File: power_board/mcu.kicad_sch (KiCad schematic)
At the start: 23 parts, among them J1 Conn_ARM_SWD_TagConnect_TC203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, U15 SM05B-GHS-TB(LF)(SN), U2 LM66100DCKR, U3 STM32L431KCUx

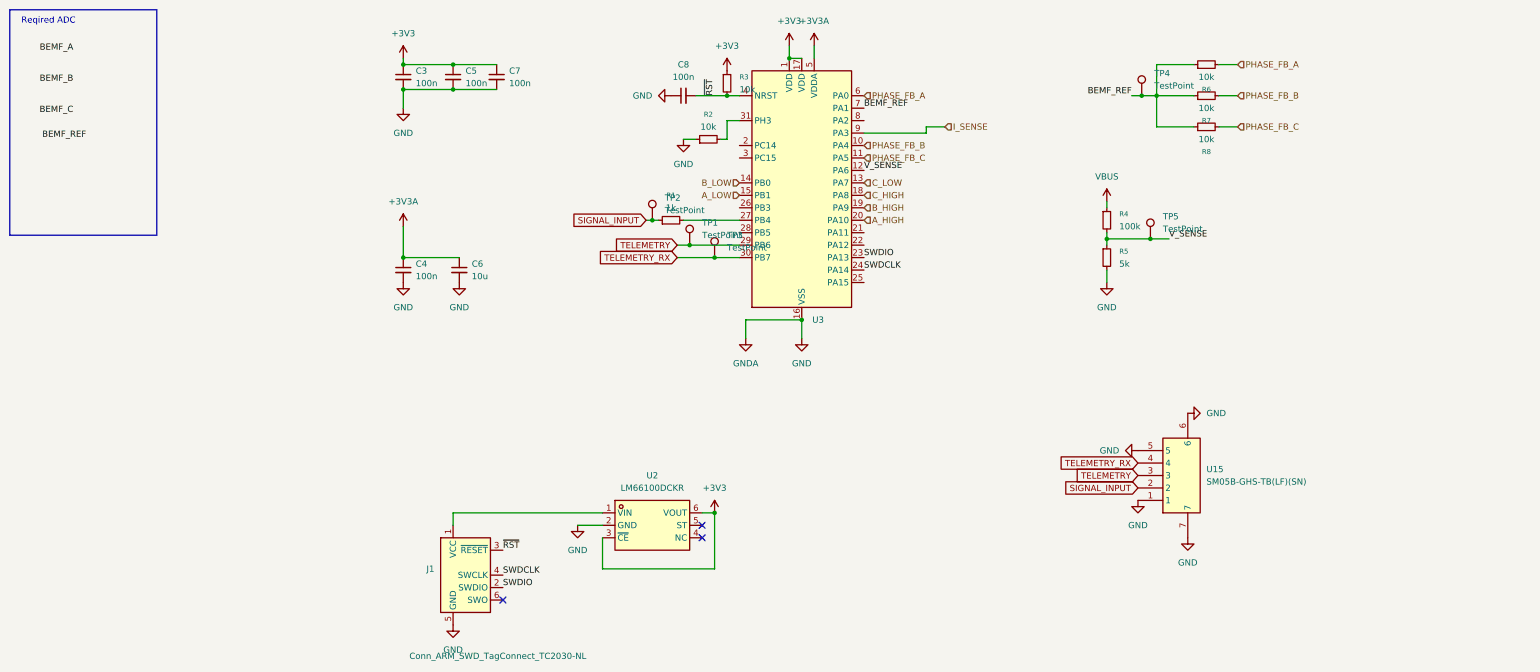
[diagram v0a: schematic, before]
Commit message: Complete all design, pass DRC
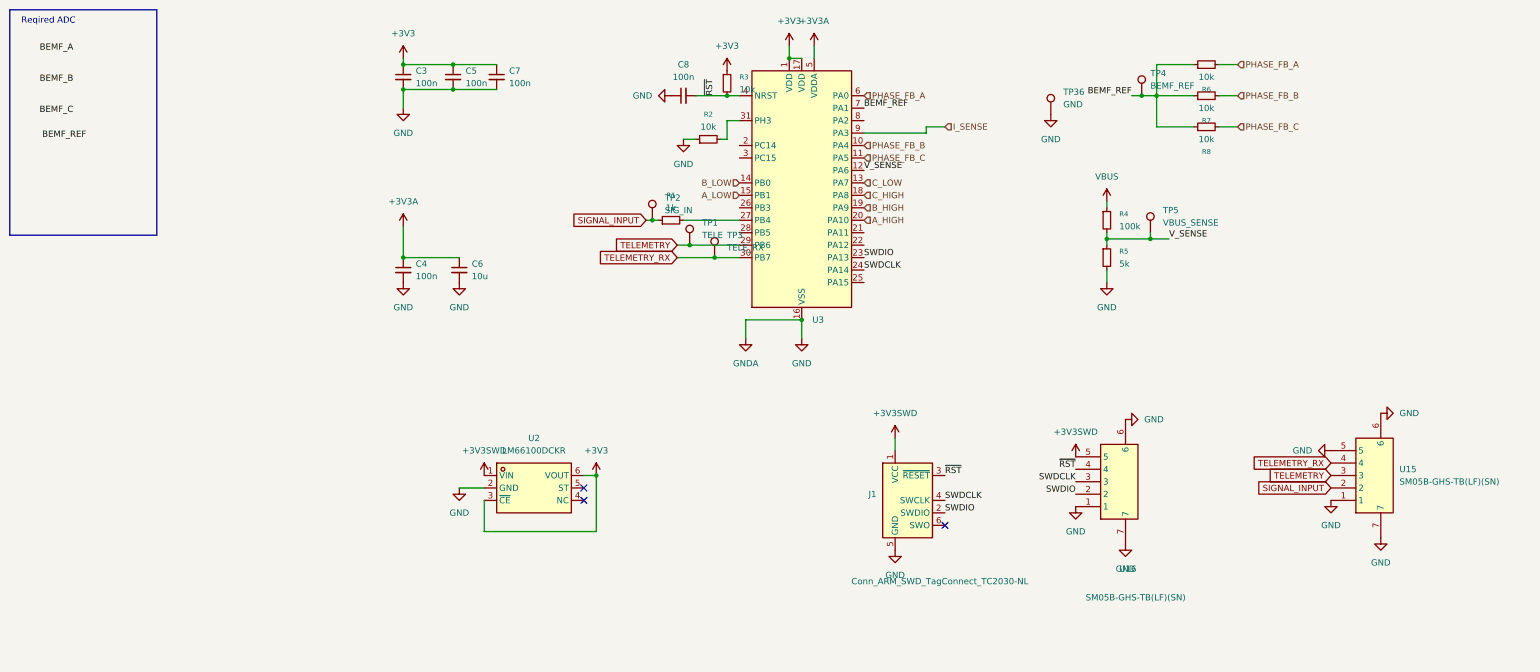
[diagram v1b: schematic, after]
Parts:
- added TP36: GND, esc-library:SMD_RH-5015, symbol Connector:TestPoint
- added U16: SM05B-GHS-TB(LF)(SN), esc-library:CONN-SMD_5P-P1.25_SM05B-GHS-TB-LF-SN, symbol esc-library:SM05B-GHS-TB(LF)(SN)
- TP1: value TestPoint -> TELE
- TP2: value TestPoint -> SIG_IN
- TP3: value TestPoint -> TELE_RX
- TP4: value TestPoint -> BEMF_REF
- TP5: value TestPoint -> VBUS_SENSE
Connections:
- net GND: now also TP36.1, U16.1, U16.6, U16.7
- net SWDCLK: now also U16.3
- net SWDIO: now also U16.2
- net ~{RST}: now also U16.4
- net +3V3SWD: now reaches J1.1 (VCC), U2.1 (VIN)
- net +3V3SWD: now also U16.5
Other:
- moved on the sheet: J1, TP5, U15, U2
